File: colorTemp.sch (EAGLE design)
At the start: 29 parts, among them IC1 STM32F10XCXT6, IC3 AOZ1284PI

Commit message: Supply change
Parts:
- removed C11, C12: 1n, blebox-rcl:C0402
- removed C14, C15, C17: 100n, blebox-rcl:C0402
- removed C18, C21: 10u, rcl:C-EUC1206
- removed C19: 220u/4V, rcl:CPOL-EUSMCC
- removed C2: 100u/25V, blebox-capacitor:CPOL-E12-6
- removed D4, D8: SS14L, blebox-diode:SS14L
- removed IC3: AOZ1284PI, blebox-ao:AOZ1284PI
- removed L4: 4.7uH, EAGLE-POWER_MAGNETICS-rev17a:WE-LQS_3015
- removed R23: 100k, blebox-rcl:R0402
- removed R24: 33k, blebox-rcl:R0402
- removed R25, R27: 47k, blebox-rcl:R0402
- removed R26, R28: 10k, blebox-rcl:R0402
- added JP5: (no value), pinhead:PINHD-1X2
- added R5: (no value), rcl:R-EU_R0402
- added T1: BP103, opto-trans-siemens:BP103
- JP1: device pinhead:PINHD-1X2 -> pinhead:PINHD-1X3
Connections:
- removed net BST: C14.1, IC3.BST
- removed net COMP2: C12.1, IC3.COMP
- removed net COMPA: C12.2, R26.2
- removed net EN: IC3.EN, R27.2, R28.1
- removed net FB: IC3.FB, R23.1, R24.2
- removed net FSW: IC3.FSW, R25.2
- removed net LX: C14.2, D4.C, IC3.LX, L4.1
- removed net N$27: C15.1, C18.1, C2.+, D8.C, IC3.VIN, R27.1
- removed net SS: C11.1, IC3.SS
- removed net VIN: C21.1, D8.A
- new net ADC1: R5.1, T1.C
- new net N$19: R5.2
- new net N$25: JP5.1
- net 3V3: no longer C17.1, C19.+, L4.2, R23.2
- net GND: now also JP1.3, JP5.2, T1.E; no longer C11.2, C15.2, C17.2, C18.2, C19.-, C2.-, C21.2, D4.A, IC3.GND, R24.1, R25.1, R26.1, R28.2
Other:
- note added: "Złącze zasilania"
- note removed: "Nominal Vout: 0.8V(1+100kOhm/33kOhm) = 3.22V"
- note removed: "Pewnie jeszcze GND i ?"

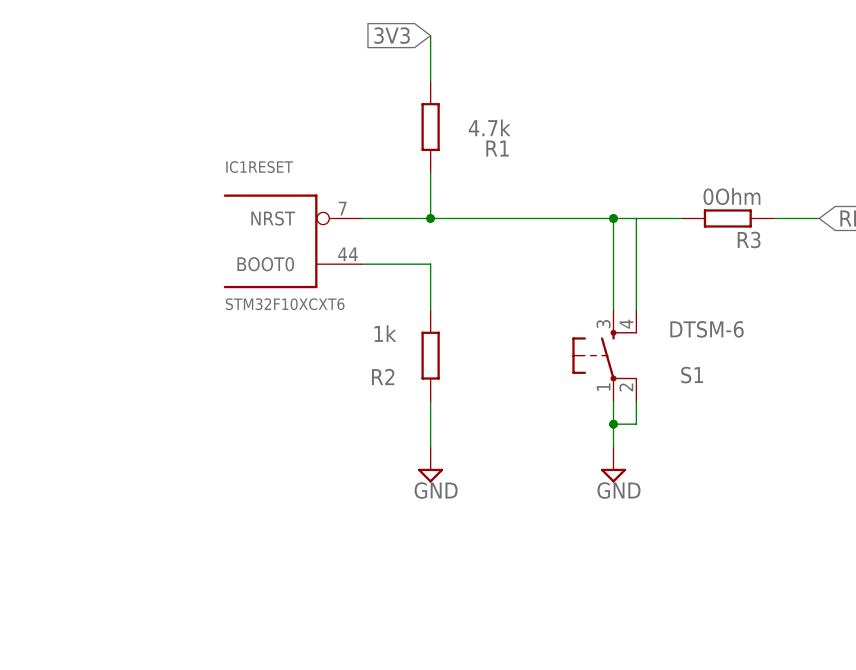
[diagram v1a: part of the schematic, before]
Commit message: Update
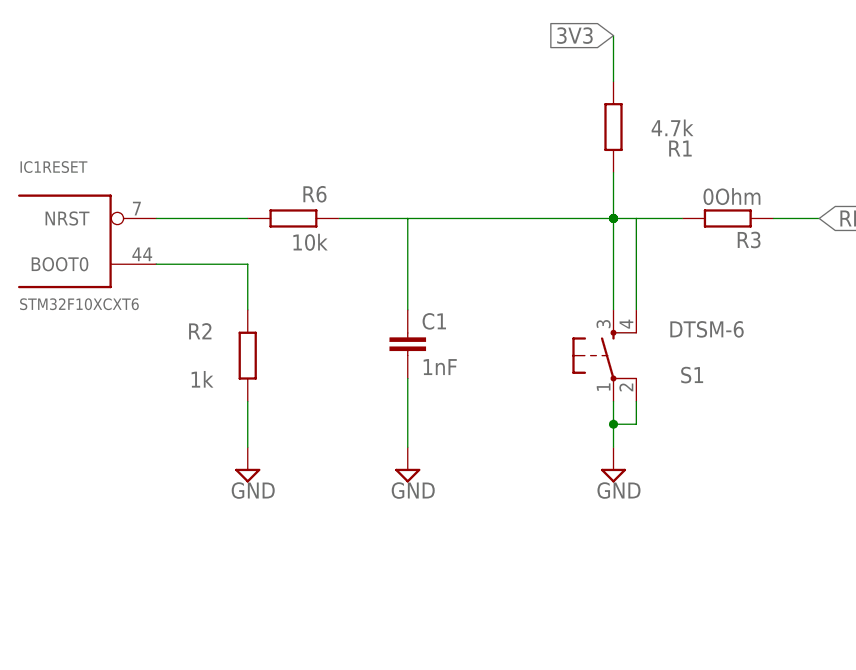
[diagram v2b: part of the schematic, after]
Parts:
- added C1: 1nF, rcl:C-EUC0402
- added R6: 10k, rcl:R-EU_R0402
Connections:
- removed net N$1: IC1RESET.NRST, R1.1, R3.2, S1.3, S1.4
- new net N$18: IC1RESET.NRST, R6.2
- new net N$20: C1.1, R1.1, R3.2, R6.1, S1.3, S1.4
- net GND: now also C1.2
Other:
- moved on the sheet: IC1RESET, R1, R2
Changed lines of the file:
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@@
 <part name="R5" library="rcl" library_urn="urn:adsk.eagle:library:334" deviceset="R-EU_" device="R0402" package3d_urn="urn:adsk.eagle:package:23547/3"/>
 <part name="SUPPLY10" library="supply2" library_urn="urn:adsk.eagle:library:372" deviceset="GND" device=""/>
+<part name="R6" library="rcl" library_urn="urn:adsk.eagle:library:334" deviceset="R-EU_" device="R0402" package3d_urn="urn:adsk.eagle:package:23547/3" value="10k"/>
+<part name="C1" library="rcl" library_urn="urn:adsk.eagle:library:334" deviceset="C-EU" device="C0402" package3d_urn="urn:adsk.eagle:package:23626/2" value="1nF"/>
+<part name="SUPPLY11" library="supply2" library_urn="urn:adsk.eagle:library:372" deviceset="GND" device=""/>
 </parts>
 <sheets>
@@
 <attribute name="NAME" x="152.4" y="71.12" size="1.27" layer="95"/>
 </instance>
-<instance part="IC1" gate="RESET" x="30.48" y="63.5" smashed="yes">
-<attribute name="VALUE" x="25.4" y="55.88" size="1.27" layer="95"/>
-<attribute name="NAME" x="25.4" y="71.12" size="1.27" layer="95"/>
-</instance>
-<instance part="R1" gate="G$1" x="48.26" y="76.2" smashed="yes" rot="R90">
-<attribute name="NAME" x="57.15" y="74.7014" size="1.778" layer="95" rot="R180"/>
-<attribute name="VALUE" x="57.15" y="76.962" size="1.778" layer="96" rot="R180"/>
-</instance>
-<instance part="R2" gate="G$1" x="48.26" y="50.8" smashed="yes" rot="R90">
-<attribute name="NAME" x="44.45" y="49.3014" size="1.778" layer="95" rot="R180"/>
-<attribute name="VALUE" x="44.45" y="54.102" size="1.778" layer="96" rot="R180"/>
+<instance part="IC1" gate="RESET" x="7.62" y="63.5" smashed="yes">
+<attribute name="VALUE" x="2.54" y="55.88" size="1.27" layer="95"/>
+<attribute name="NAME" x="2.54" y="71.12" size="1.27" layer="95"/>
+</instance>
+<instance part="R1" gate="G$1" x="68.58" y="76.2" smashed="yes" rot="R90">
+<attribute name="NAME" x="77.47" y="74.7014" size="1.778" layer="95" rot="R180"/>
+<attribute name="VALUE" x="77.47" y="76.962" size="1.778" layer="96" rot="R180"/>
+</instance>
+<instance part="R2" gate="G$1" x="27.94" y="50.8" smashed="yes" rot="R90">
+<attribute name="NAME" x="24.13" y="54.3814" size="1.778" layer="95" rot="R180"/>
+<attribute name="VALUE" x="24.13" y="49.022" size="1.778" layer="96" rot="R180"/>
 </instance>
 <instance part="S1" gate="G$1" x="68.58" y="50.8" smashed="yes">
@@
 <attribute name="VALUE" x="83.185" y="54.61" size="1.778" layer="96" rot="R180"/>
 </instance>
-<instance part="SUPPLY1" gate="GND" x="48.26" y="38.1" smashed="yes">
-<attribute name="VALUE" x="46.355" y="34.925" size="1.778" layer="96"/>
+<instance part="SUPPLY1" gate="GND" x="27.94" y="38.1" smashed="yes">
+<attribute name="VALUE" x="26.035" y="34.925" size="1.778" layer="96"/>
 </instance>
 <instance part="SUPPLY2" gate="GND" x="68.58" y="38.1" smashed="yes">
@@
 <instance part="SUPPLY10" gate="GND" x="58.42" y="-114.3" smashed="yes">
 <attribute name="VALUE" x="59.055" y="-112.395" size="1.778" layer="96"/>
+</instance>
+<instance part="R6" gate="G$1" x="33.02" y="66.04" smashed="yes" rot="R180">
+<attribute name="NAME" x="36.83" y="69.6214" size="1.778" layer="95" rot="R180"/>
+<attribute name="VALUE" x="36.83" y="64.262" size="1.778" layer="96" rot="R180"/>
+</instance>
+<instance part="C1" gate="G$1" x="45.72" y="53.34" smashed="yes">
+<attribute name="NAME" x="47.244" y="53.721" size="1.778" layer="95"/>
+<attribute name="VALUE" x="47.244" y="48.641" size="1.778" layer="96"/>
+</instance>
+<instance part="SUPPLY11" gate="GND" x="45.72" y="38.1" smashed="yes">
+<attribute name="VALUE" x="43.815" y="34.925" size="1.778" layer="96"/>
 </instance>
 </instances>
@@
 </busses>
 <nets>
-<net name="N$1" class="0">
-<segment>
-<pinref part="IC1" gate="RESET" pin="NRST"/>
-<wire x1="40.64" y1="66.04" x2="48.26" y2="66.04" width="0.1524" layer="91"/>
-<pinref part="R1" gate="G$1" pin="1"/>
-<wire x1="48.26" y1="66.04" x2="48.26" y2="71.12" width="0.1524" layer="91"/>
-<pinref part="S1" gate="G$1" pin="3"/>
-<wire x1="48.26" y1="66.04" x2="68.58" y2="66.04" width="0.1524" layer="91"/>
-<wire x1="68.58" y1="66.04" x2="68.58" y2="55.88" width="0.1524" layer="91"/>
-<pinref part="S1" gate="G$1" pin="4"/>
-<wire x1="71.12" y1="55.88" x2="71.12" y2="66.04" width="0.1524" layer="91"/>
-<wire x1="71.12" y1="66.04" x2="68.58" y2="66.04" width="0.1524" layer="91"/>
-<junction x="48.26" y="66.04"/>
-<junction x="68.58" y="66.04"/>
-<pinref part="R3" gate="G$1" pin="2"/>
-<wire x1="71.12" y1="66.04" x2="76.2" y2="66.04" width="0.1524" layer="91"/>
-</segment>
-</net>
 <net name="N$2" class="0">
 <segment>
 <pinref part="IC1" gate="RESET" pin="BOOT0"/>
-<wire x1="40.64" y1="60.96" x2="48.26" y2="60.96" width="0.1524" layer="91"/>
+<wire x1="17.78" y1="60.96" x2="27.94" y2="60.96" width="0.1524" layer="91"/>
 <pinref part="R2" gate="G$1" pin="2"/>
-<wire x1="48.26" y1="60.96" x2="48.26" y2="55.88" width="0.1524" layer="91"/>
+<wire x1="27.94" y1="60.96" x2="27.94" y2="55.88" width="0.1524" layer="91"/>
 </segment>
 </net>
@@
 <pinref part="R2" gate="G$1" pin="1"/>
 <pinref part="SUPPLY1" gate="GND" pin="GND"/>
-<wire x1="48.26" y1="45.72" x2="48.26" y2="40.64" width="0.1524" layer="91"/>
+<wire x1="27.94" y1="45.72" x2="27.94" y2="40.64" width="0.1524" layer="91"/>
 </segment>
 <segment>
@@
 <wire x1="58.42" y1="-111.76" x2="58.42" y2="-109.22" width="0.1524" layer="91"/>
 </segment>
+<segment>
+<pinref part="C1" gate="G$1" pin="2"/>
+<pinref part="SUPPLY11" gate="GND" pin="GND"/>
+<wire x1="45.72" y1="48.26" x2="45.72" y2="40.64" width="0.1524" layer="91"/>
+</segment>
 </net>
 <net name="3V3" class="0">
 <segment>
 <pinref part="R1" gate="G$1" pin="2"/>
-<wire x1="48.26" y1="81.28" x2="48.26" y2="86.36" width="0.1524" layer="91"/>
-<label x="48.26" y="86.36" size="1.778" layer="95" rot="R180" xref="yes"/>
+<wire x1="68.58" y1="81.28" x2="68.58" y2="86.36" width="0.1524" layer="91"/>
+<label x="68.58" y="86.36" size="1.778" layer="95" rot="R180" xref="yes"/>
 <label x="172.72" y="83.82" size="1.778" layer="95" rot="R180" xref="yes"/>
 <label x="142.24" y="-25.4" size="1.778" layer="95" rot="R180" xref="yes"/>
@@
 </segment>
 </net>
+<net name="N$18" class="0">
+<segment>
+<pinref part="IC1" gate="RESET" pin="NRST"/>
+<pinref part="R6" gate="G$1" pin="2"/>
+<wire x1="17.78" y1="66.04" x2="27.94" y2="66.04" width="0.1524" layer="91"/>
+</segment>
+</net>
+<net name="N$20" class="0">
+<segment>
+<pinref part="R6" gate="G$1" pin="1"/>
+<wire x1="38.1" y1="66.04" x2="45.72" y2="66.04" width="0.1524" layer="91"/>
+<pinref part="C1" gate="G$1" pin="1"/>
+<wire x1="45.72" y1="66.04" x2="45.72" y2="55.88" width="0.1524" layer="91"/>
+<pinref part="R1" gate="G$1" pin="1"/>
+<wire x1="68.58" y1="66.04" x2="68.58" y2="71.12" width="0.1524" layer="91"/>
+<pinref part="S1" gate="G$1" pin="3"/>
+<wire x1="68.58" y1="66.04" x2="68.58" y2="55.88" width="0.1524" layer="91"/>
+<pinref part="S1" gate="G$1" pin="4"/>
+<wire x1="71.12" y1="55.88" x2="71.12" y2="66.04" width="0.1524" layer="91"/>
+<wire x1="71.12" y1="66.04" x2="68.58" y2="66.04" width="0.1524" layer="91"/>
+<junction x="68.58" y="66.04"/>
+<junction x="68.58" y="66.04"/>
+<pinref part="R3" gate="G$1" pin="2"/>
+<wire x1="71.12" y1="66.04" x2="76.2" y2="66.04" width="0.1524" layer="91"/>
+<wire x1="45.72" y1="66.04" x2="68.58" y2="66.04" width="0.1524" layer="91"/>
+</segment>
+</net>

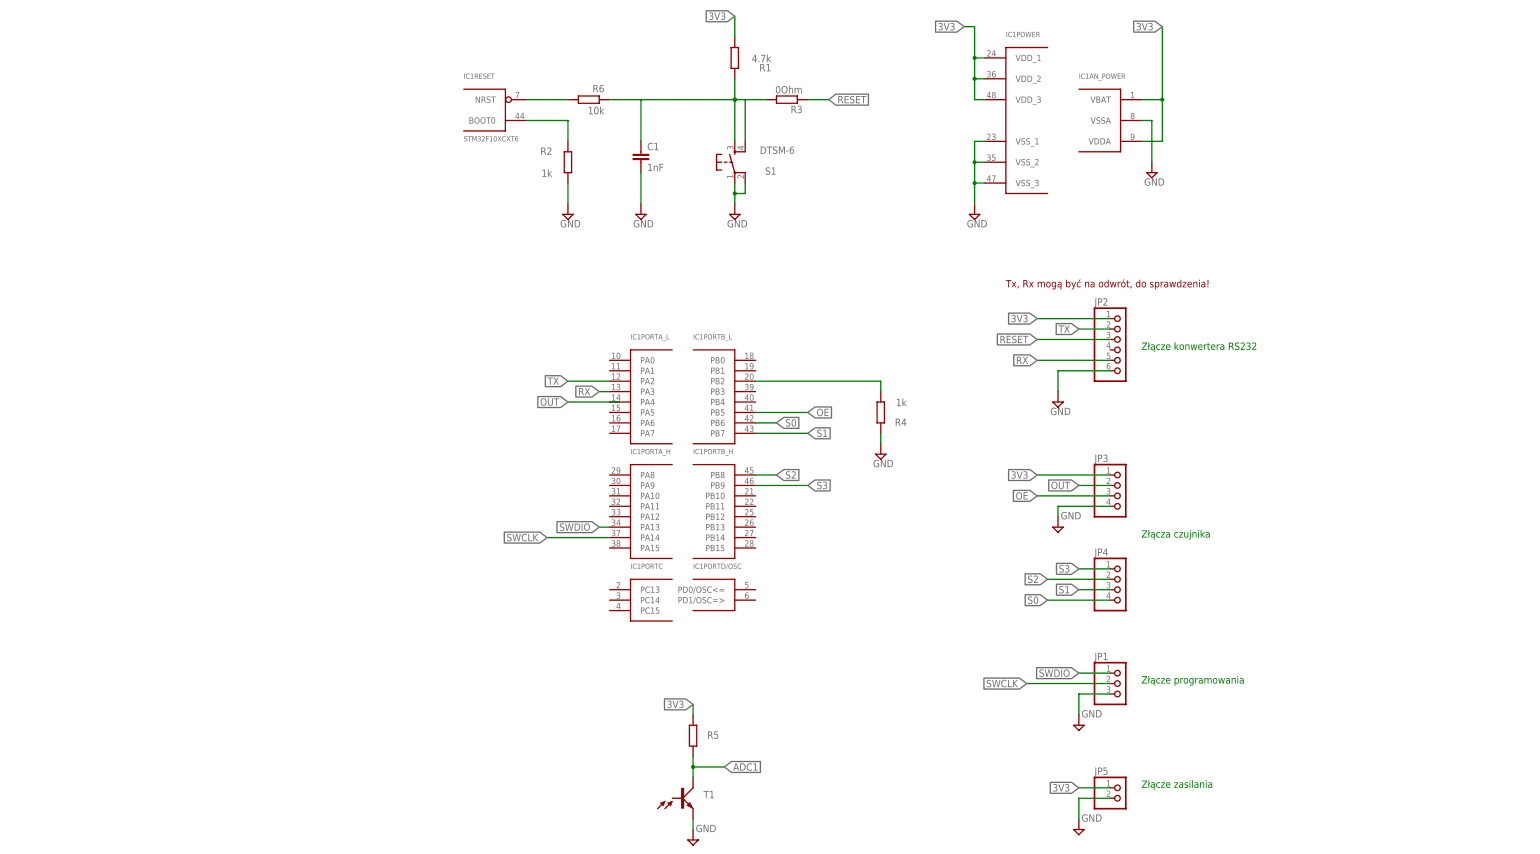
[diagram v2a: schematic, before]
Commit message: Schematic Update
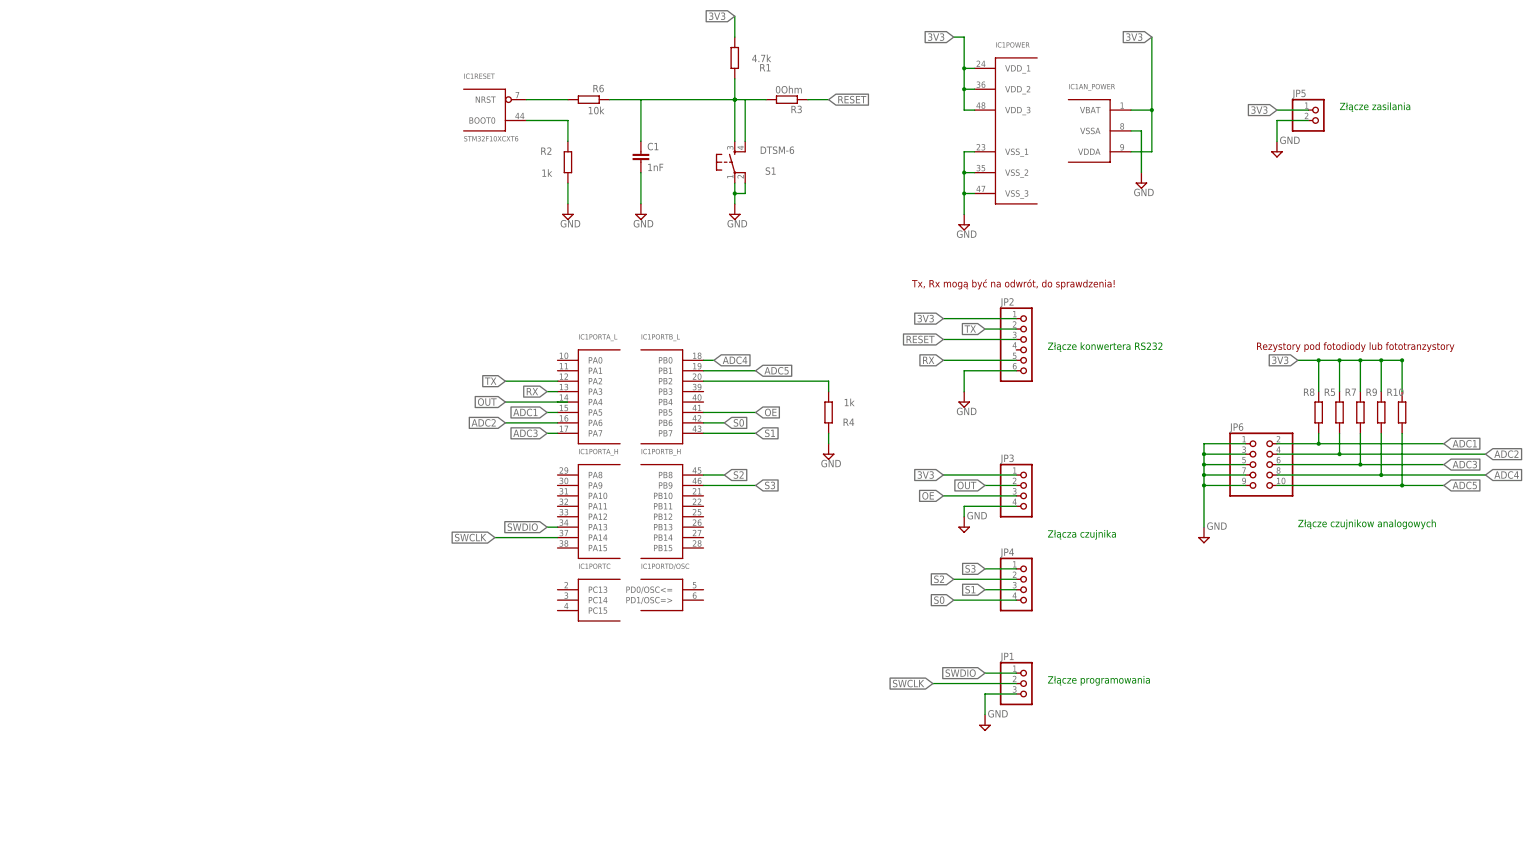
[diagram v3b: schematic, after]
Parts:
- removed T1: BP103, opto-trans-siemens:BP103
- added JP6: (no value), pinhead:PINHD-2X5
- added R10, R7, R8, R9: (no value), rcl:R-EU_R0402
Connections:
- new net ADC2: JP6.4, R5.2
- new net ADC3: JP6.6, R7.2
- new net ADC4: JP6.8, R9.2
- new net ADC5: JP6.10, R10.2
- new net N$1: R10.1, R5.1, R7.1, R8.1, R9.1
- new net N$21: IC1PORTA_L.PA5
- new net N$22: IC1PORTB_L.PB0
- new net N$23: IC1PORTA_L.PA6
- new net N$24: IC1PORTA_L.PA7
- net ADC1: now also JP6.2, R8.2; no longer R5.1, T1.C
- net GND: now also JP6.1, JP6.3, JP6.5, JP6.7, JP6.9; no longer T1.E
- net N$19: now also IC1PORTB_L.PB1; no longer R5.2
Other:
- note added: "Rezystory pod fotodiody lub fototranzystory"
- note added: "Złącze czujnikow analogowych"
- moved on the sheet: IC1AN_POWER, IC1PORTA_H, IC1PORTA_L, IC1PORTB_H, IC1PORTB_L, IC1PORTC, IC1PORTD/OSC, IC1POWER, JP1, JP2, JP3, JP4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
